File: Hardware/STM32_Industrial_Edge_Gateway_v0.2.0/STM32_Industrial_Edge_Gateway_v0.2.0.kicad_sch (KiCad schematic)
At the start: 25 parts, among them J1 DC Power Jack (5.5 x 2.1mm), Q1 IRLML6402, U1 MP2338GTL-Z, U2 TLV76733DRVx

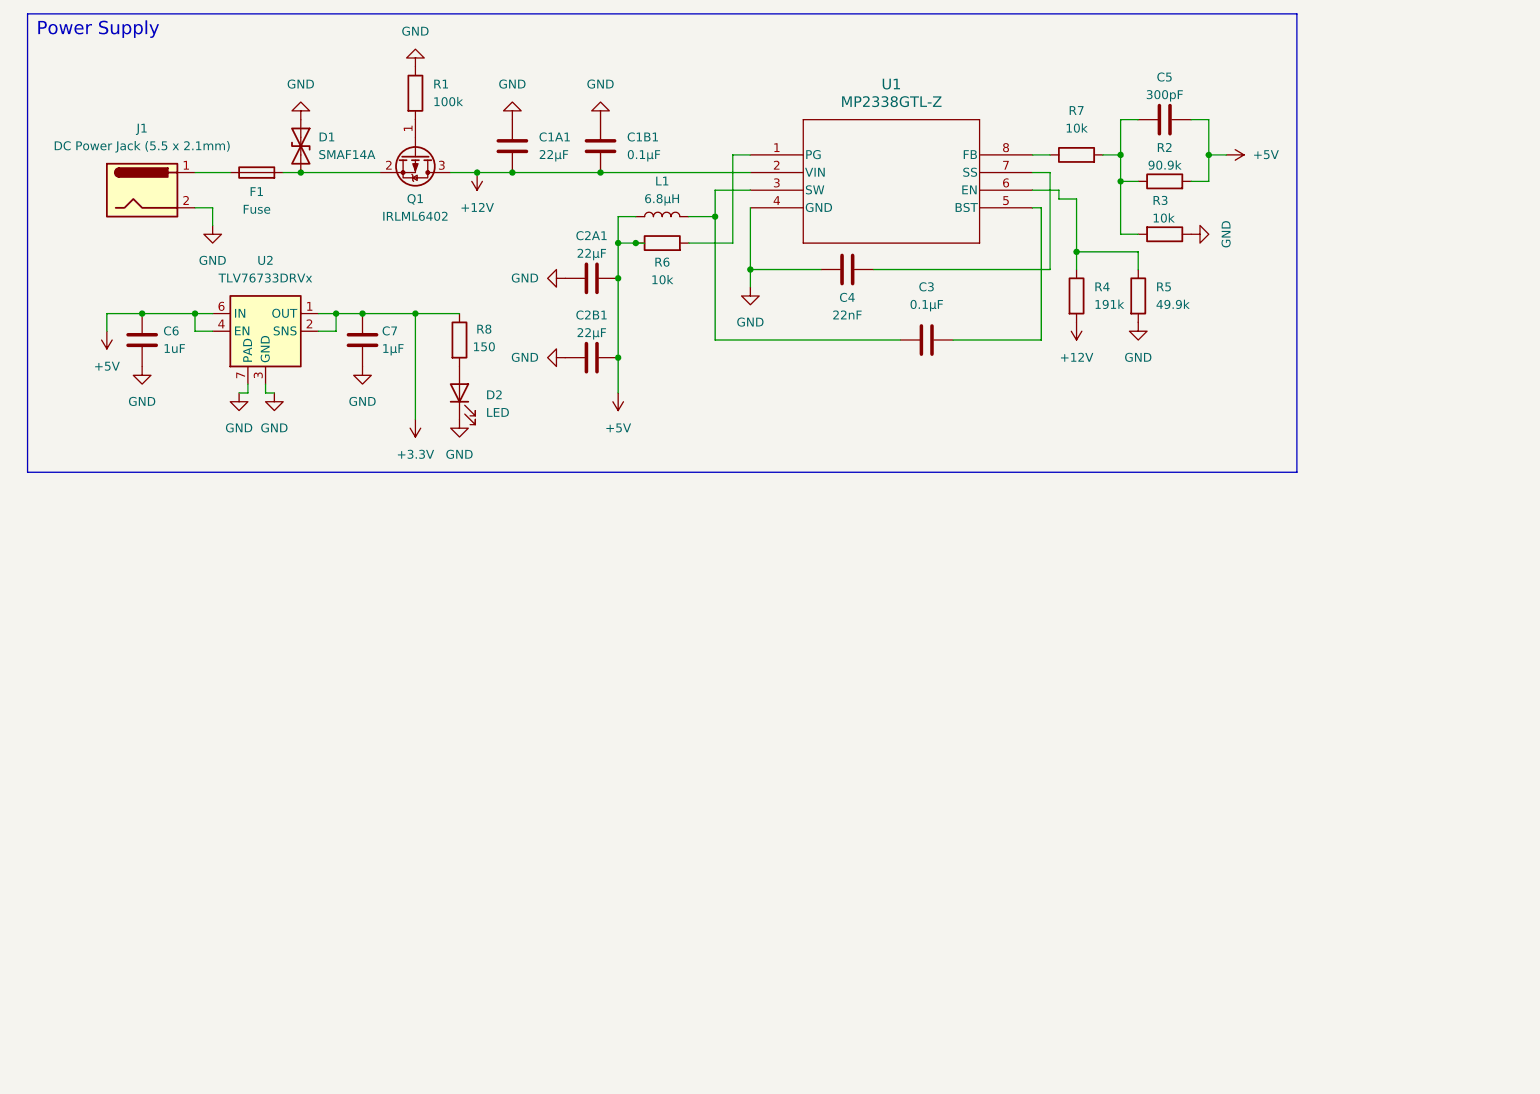
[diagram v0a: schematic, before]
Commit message: STM32 MCU Core Schematic
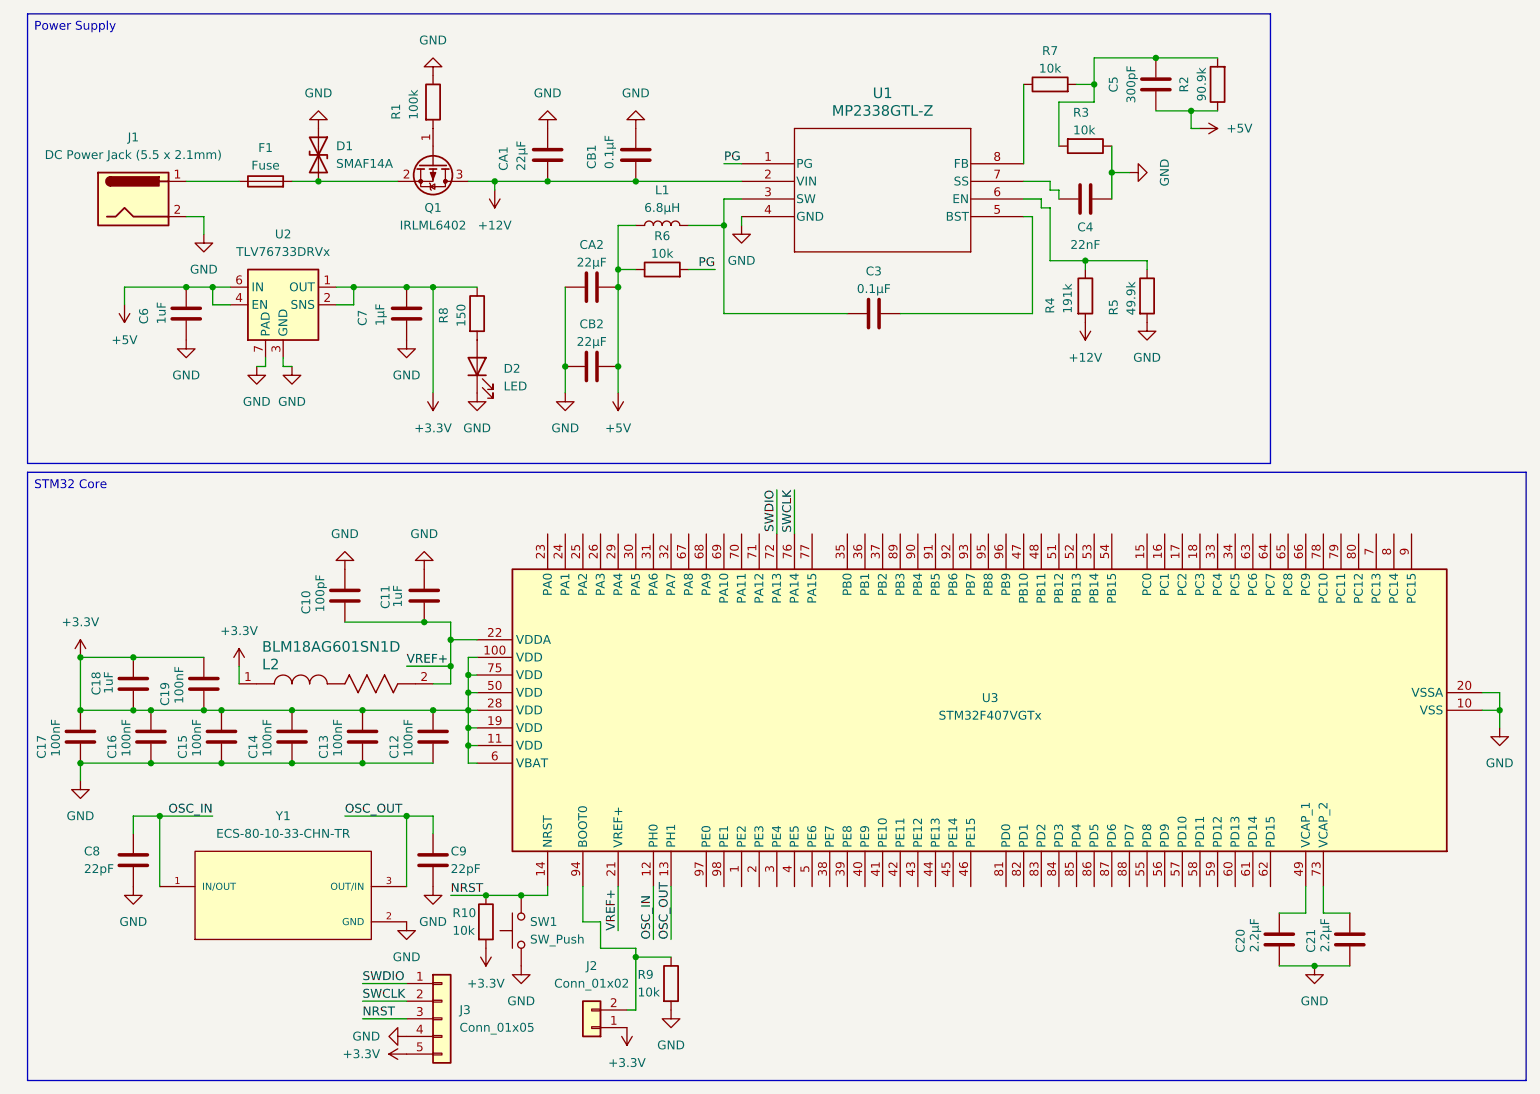
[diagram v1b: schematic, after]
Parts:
- added C10: 100pF, symbol Device:C
- added C11, C18: 1uF, symbol Device:C
- added C12, C13, C14, C15, C16, C17, C19: 100nF, symbol Device:C
- added C20, C21: 2.2µF, symbol Device:C
- added C8, C9: 22pF, symbol Device:C
- added J2: Conn_01x02, symbol Connector_Generic:Conn_01x02
- added J3: Conn_01x05, symbol Connector_Generic:Conn_01x05
- added L2: BLM18AG601SN1D, FILTER_BLM18AG_MUR, symbol BLM18AG601SN1D:BLM18AG601SN1D
- added R10, R9: 10k, symbol Device:R
- added SW1: SW_Push, symbol Switch:SW_Push
- added U3: STM32F407VGTx, Package_QFP:LQFP-100_14x14mm_P0.5mm, symbol MCU_ST_STM32F4:STM32F407VGTx
- added Y1: ECS-80-10-33-CHN-TR, ECS-80-10-33-CHN-TR:XTAL_ECS-80-10-33-CHN-TR, symbol ECS-80-10-33-CHN-TR:ECS-80-10-33-CHN-TR
- renumbered C1A1 to CA1, C2A1 to CA2, C1B1 to CB1, C2B1 to CB2
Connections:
- net +3.3V: now also C12.1, C13.1, C14.1, C15.1, C16.1, C17.1, C18.1, C18.2, C19.1, C19.2, J2.1 (Pin_1), J3.5 (Pin_5), L2.1, R10.2, U3.100 (VDD), U3.11 (VDD), U3.19 (VDD), U3.28 (VDD), U3.50 (VDD), U3.6 (VBAT), U3.75 (VDD)
- net +5V: now also C5.1, R2.1; no longer C5.2, R2.2
- net GND: now also C4.2, C10.1, C11.1, C12.2, C13.2, C14.2, C15.2, C16.2, C17.2, C20.2, C21.2, C8.1, C9.1, J3.4 (Pin_4), R9.2, SW1.1, U3.10 (VSS), U3.20 (VSSA), U3.27 (VSS), U3.74 (VSS), U3.99 (VSS), Y1.2 (GND), Y1.4 (GND); no longer C4.1
- net at R3.2, R7.2: now also C5.2, R2.2; no longer C5.1, R2.1
- net PG: now reaches R6.2, U1.1 (PG)
- net at U1.7 (SS): now also C4.1; no longer C4.2
- new net: C21.1, U3.73 (VCAP_2)
- new net: J2.2 (Pin_2), R9.1, U3.94 (BOOT0)
- new net: C20.1, U3.49 (VCAP_1)
- new net NRST: J3.3 (Pin_3), R10.1, SW1.2, U3.14 (NRST)
- new net OSC_IN: C8.2, U3.12 (PH0), Y1.1 (IN/OUT)
- new net OSC_OUT: C9.2, U3.13 (PH1), Y1.3 (OUT/IN)
- new net SWCLK: J3.2 (Pin_2), U3.76 (PA14)
- new net SWDIO: J3.1 (Pin_1), U3.72 (PA13)
- new net VREF+: C10.2, C11.2, L2.2, U3.21 (VREF+), U3.22 (VDDA)
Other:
- note removed: "Power Supply"
- title: STM32 Industrial Edge Gateway -> STM32 Industrial Edge Gateway - v0.2.0
- moved on the sheet: C3, C4, C5, C6, C7, CA1, CA2, CB1, CB2, D1, D2, F1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
